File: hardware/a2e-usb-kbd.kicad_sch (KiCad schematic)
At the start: 10 parts, among them J1 Apple IIe KBD Connector, U1 CD74HC4067M, U2 74HC4051

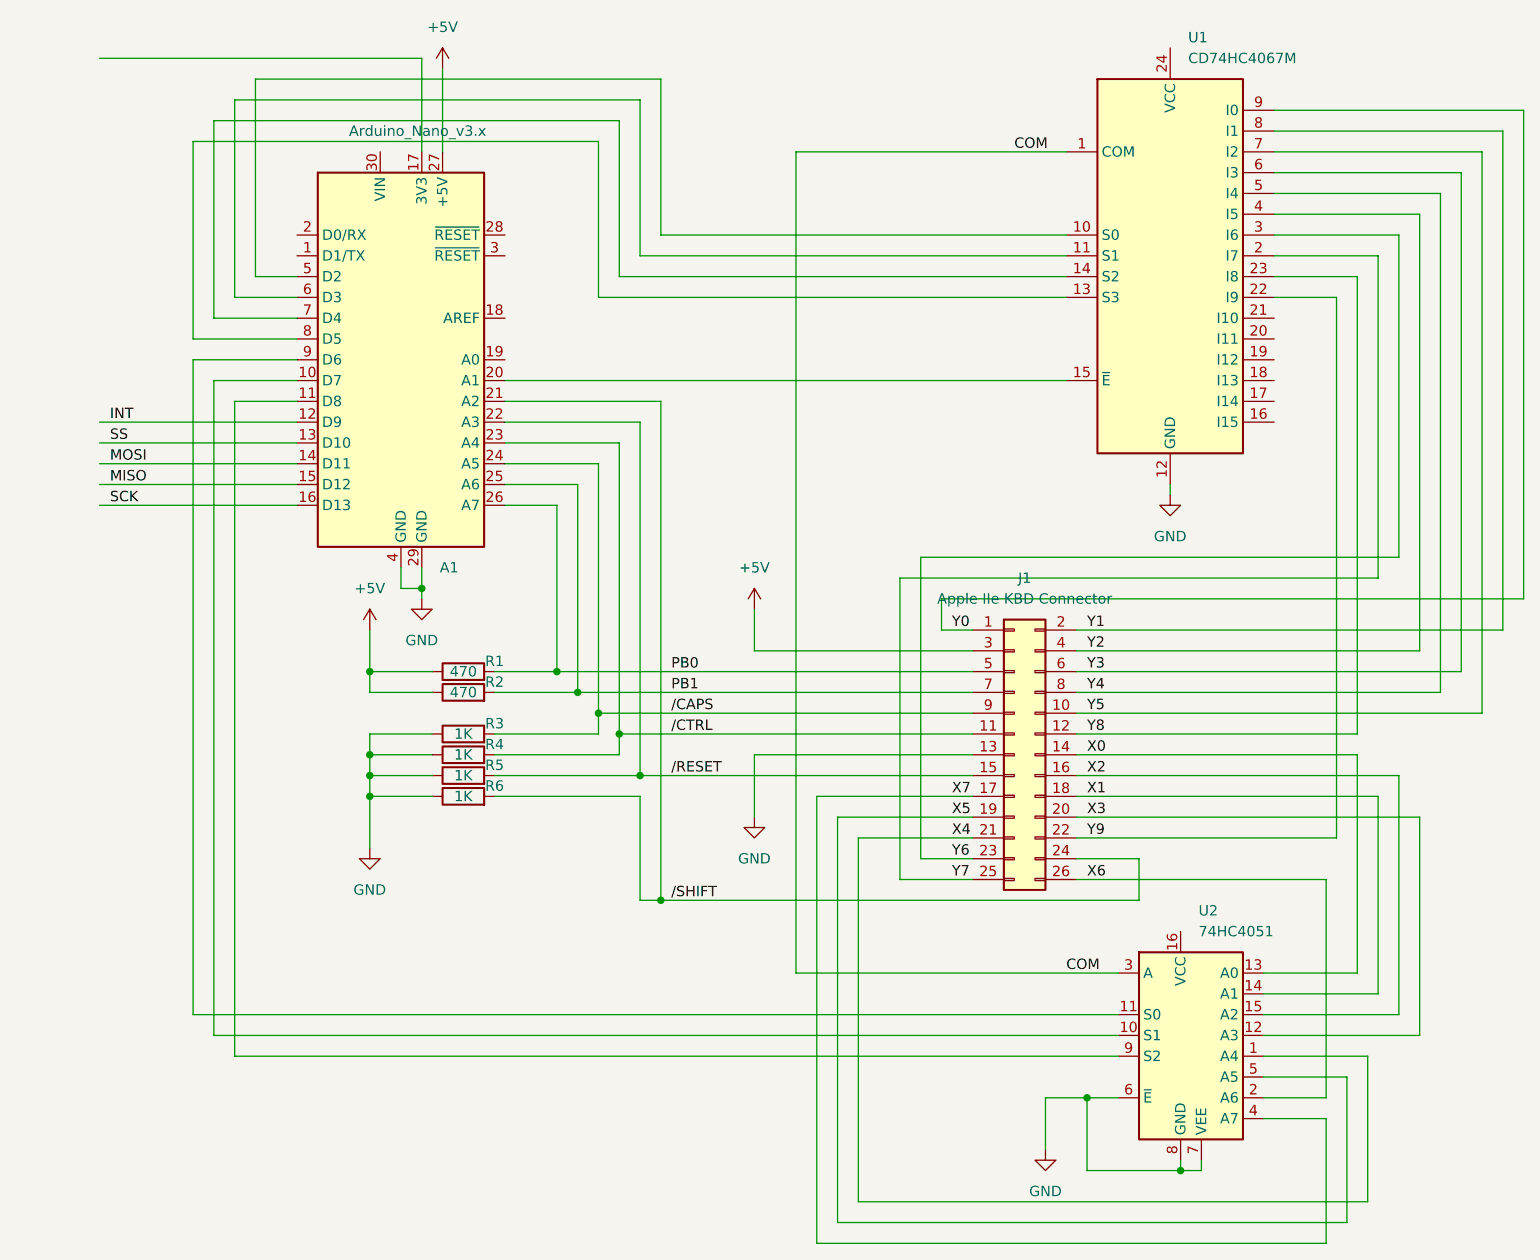
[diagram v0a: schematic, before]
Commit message: update schematics
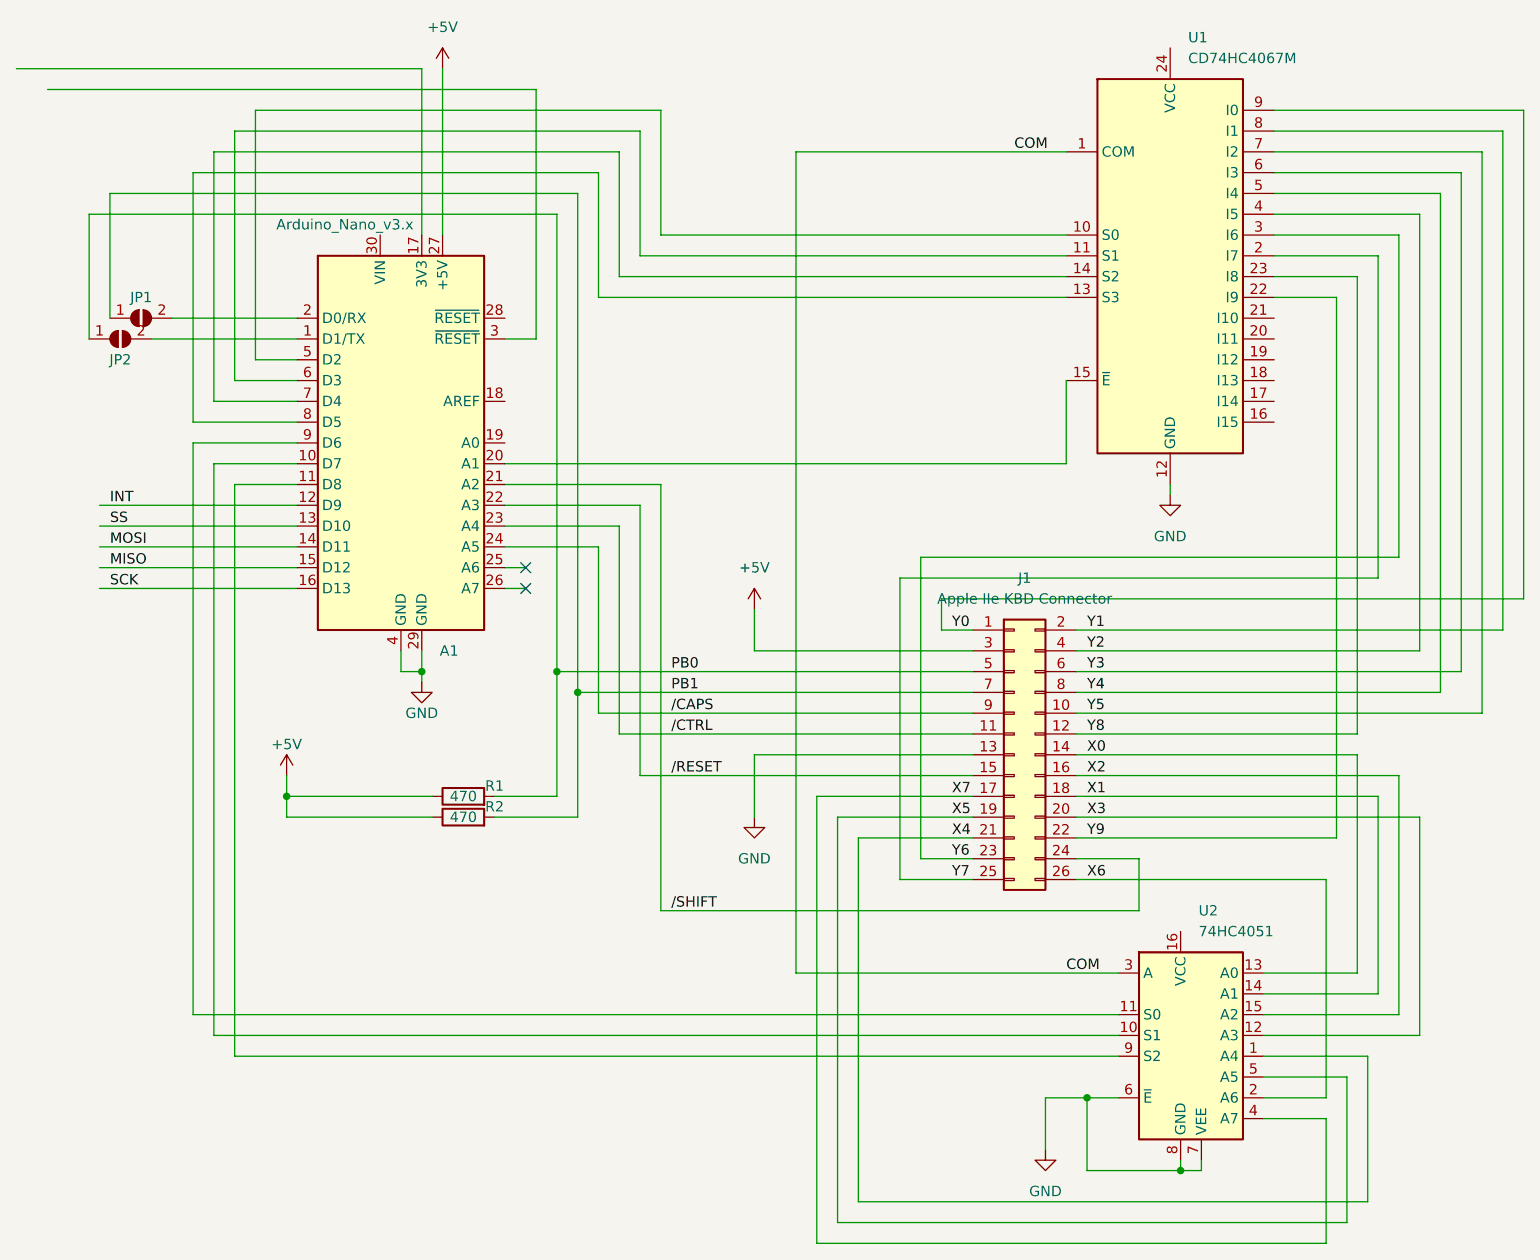
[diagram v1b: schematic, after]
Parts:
- removed R3, R4, R5, R6: 1K, symbol Device:R
- added JP1, JP2: SolderJumper_2_Open, symbol Jumper:SolderJumper_2_Open
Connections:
- net PB0: now also JP2.1 (A); no longer A1.26 (A7)
- net PB1: now also JP1.1 (A); no longer A1.25 (A6)
- net at A1.1 (D1/TX): now also JP2.2 (B)
- net at A1.2 (D0/RX): now also JP1.2 (B)
- no-connect marks 0 -> 2
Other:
- moved on the sheet: A1, R1, R2
